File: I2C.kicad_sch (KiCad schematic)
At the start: 10 parts, among them J13 XH-4A connector, J14 2350514-8, U11 TLA2528IRTER

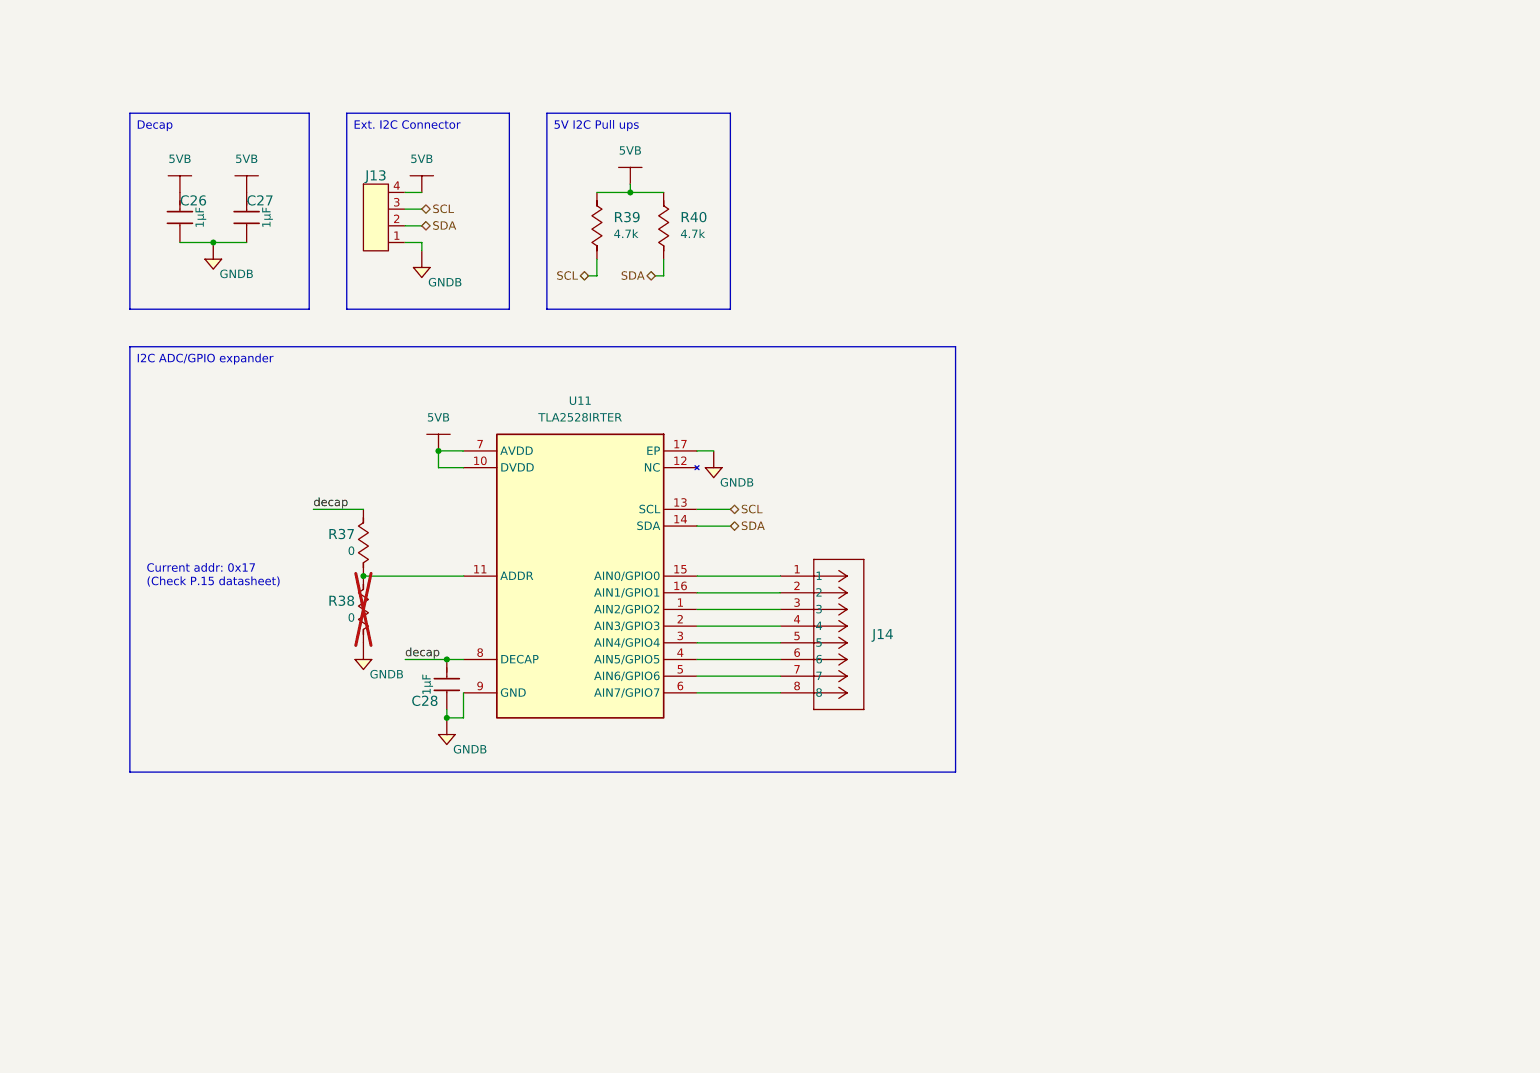
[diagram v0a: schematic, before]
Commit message: update schematique
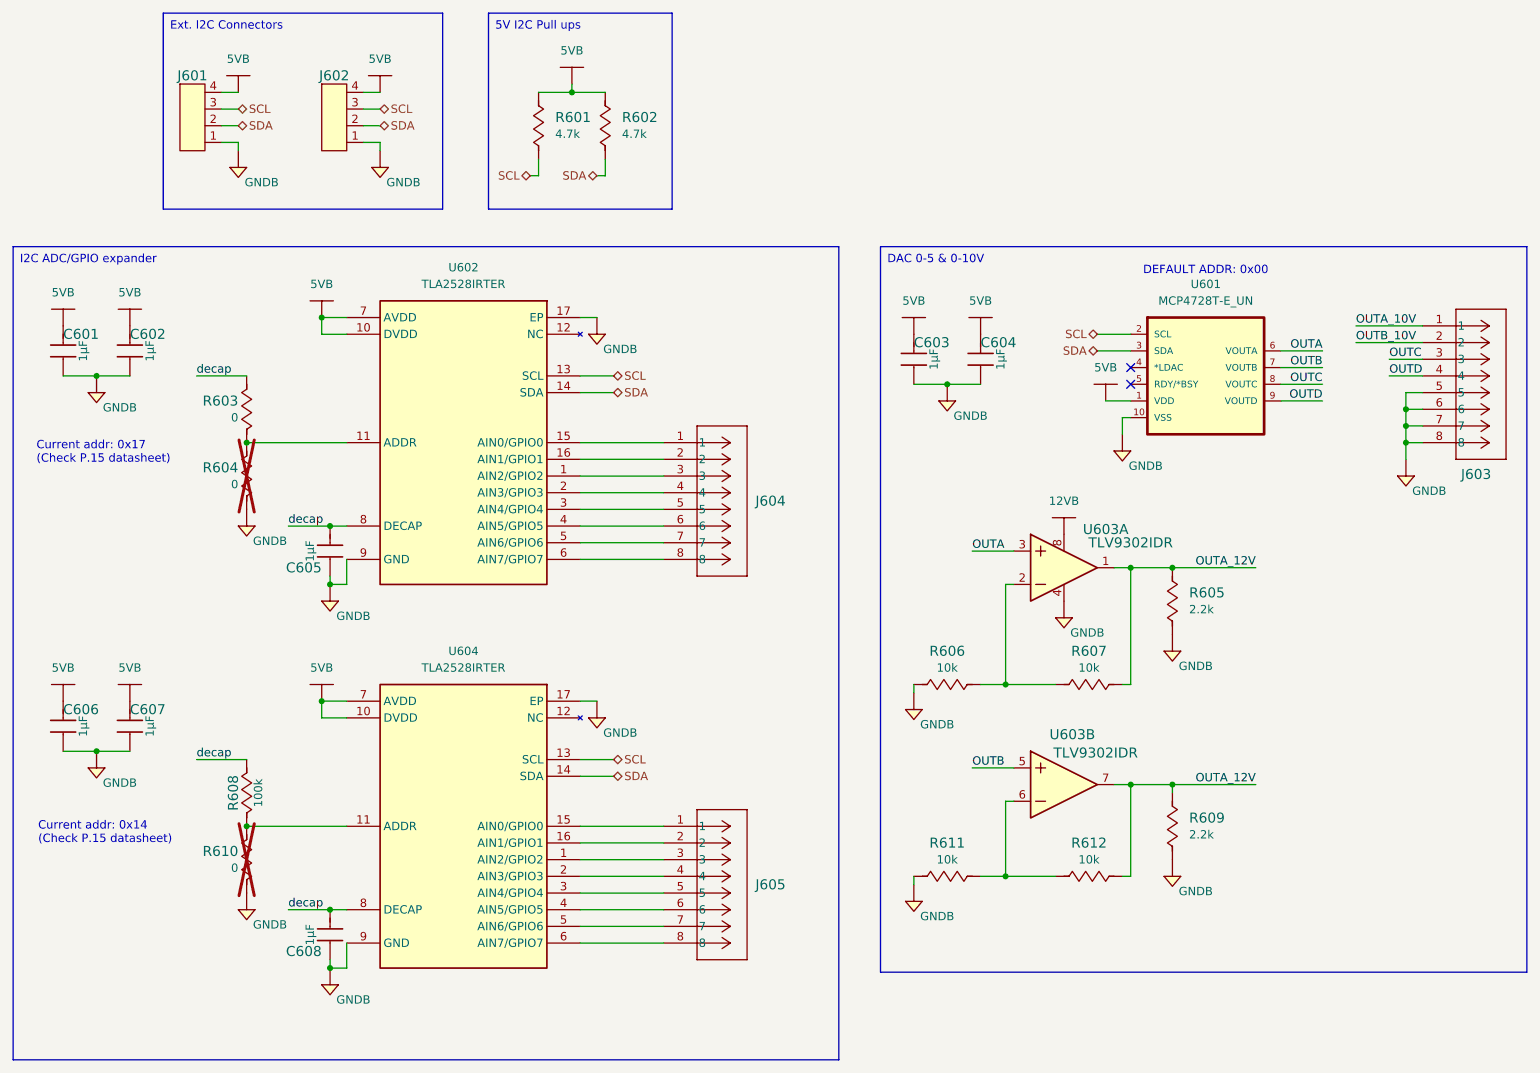
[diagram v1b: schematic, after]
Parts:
- added C603, C604, C606, C607, C608: 885012107015, Capacitors:C0603, symbol Capacitors:885012106022
- added J602: XH-4A connector, Connectors:XH-4A, symbol Connectors:XH-4A connector
- added J603, J605: 2350514-8, Connectors:CONN8_2350514-8_TEC, symbol Connectors:2350514-8
- added R605, R609: RC0805JR-072K2L, Resistors:R0805, symbol Resistors:RC0805JR-072K2L
- added R606, R607, R611, R612: RC0805JR-0710KL, Resistors:R0805, symbol Resistors:RC0805JR-0710KL
- added R608: RC0805JR-07100KL, Resistors:R0805, symbol Resistors:RC0805JR-07100KL
- added R610: RC0805JR-070RL, Resistors:R0603, symbol Resistors:RC0805JR-070RL
- added U601: MCP4728T-E_UN, IC:SOP50P490X110-10N, symbol DAC:MCP4728T-E_UN
- added U603: TLV9302IDR, Assembly:IC8_TLV9302IDR_TEX, symbol Amplifiers:TLV9302IDR
- added U604: TLA2528IRTER, QFN50P300X300X80-17N-D, symbol ADC:TLA2528IRTER
- renumbered C26 to C601, C27 to C602, C28 to C605, J13 to J601, J14 to J604, R39 to R601, R40 to R602, R37 to R603, R38 to R604, U11 to U602
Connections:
- net 5VB: now also C603.2, C604.2, C606.2, C607.2, J602.4, U601.1 (VDD), U604.10 (DVDD), U604.7 (AVDD)
- net GNDB: now also C603.1, C604.1, C606.1, C607.1, C608.1, J602.1, J603.5, J603.6, J603.7, J603.8, R605.1, R606.1, R609.1, R610.2, R611.1, U601.10 (VSS), U603.4, U604.17 (EP), U604.9 (GND)
- net SCL: now also J602.3, U601.2 (SCL), U604.13 (SCL)
- net SDA: now also J602.2, U601.3 (SDA), U604.14 (SDA)
- net decap: now also C608.2, R608.1, U604.8 (DECAP)
- new net: R611.2, R612.1, U603.6
- new net: R608.2, R610.1, U604.11 (ADDR)
- new net: R606.2, R607.1, U603.2
- new net: J605.1, U604.15 (AIN0/GPIO0)
- new net: J605.2, U604.16 (AIN1/GPIO1)
- new net: J605.3, U604.1 (AIN2/GPIO2)
- new net: J605.4, U604.2 (AIN3/GPIO3)
- new net: J605.5, U604.3 (AIN4/GPIO4)
- new net: J605.6, U604.4 (AIN5/GPIO5)
- new net: J605.7, U604.5 (AIN6/GPIO6)
- new net: J605.8, U604.6 (AIN7/GPIO7)
- new net 12VB: U603.8
- new net OUTA: U601.6 (VOUTA), U603.3
- new net OUTA_10V: J603.1
- new net OUTA_12V: R605.2, R607.2, R609.2, R612.2, U603.1, U603.7
- new net OUTB: U601.7 (VOUTB), U603.5
- new net OUTB_10V: J603.2
- new net OUTC: J603.3, U601.8 (VOUTC)
- new net OUTD: J603.4, U601.9 (VOUTD)
- no-connect marks 0 -> 2
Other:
- note added: "Current addr: 0x14 (Check P.15 datasheet)"
- note added: "DEFAULT ADDR: 0x00"
- moved on the sheet: C601, C602, C605, J601, J604, R601, R602, R603, R604, U602
